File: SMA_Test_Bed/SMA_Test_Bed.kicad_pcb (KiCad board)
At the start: 2 copper layers, 108.6 x 58.3 mm, 157 parts, among them J1 Conn_02x14_Counter_Clockwise, J10 Conn_01x02_Socket, J11 Conn_01x02_Socket, J12 Conn_01x02_Socket, J13 Conn_01x02_Socket, J14 Conn_01x02_Socket, J15 Conn_01x02_Socket, J16 Conn_01x02_Socket, J17 Conn_01x02_Socket, J18 Conn_01x02_Socket, J2 Conn_01x02_Socket, J3 Conn_01x02_Socket, J4 Conn_01x02_Socket, J5 Conn_01x02_Socket, J6 Conn_01x02_Socket, J7 Conn_01x02_Socket, J8 Conn_01x02_Socket, J9 Conn_01x02_Socket, Q1 NMOS, Q10 NMOS, Q11 NMOS, Q12 NMOS, Q13 NMOS, Q14 NMOS, Q15 NMOS, Q16 NMOS, Q2 NMOS, Q3 NMOS, Q4 NMOS, Q5 NMOS, Q6 NMOS, Q7 NMOS, Q8 NMOS, Q9 NMOS, U1 PCA9685PW, U2 TLV9044, U3 TLV9044, U4 TLV9044, U5 TLV9044

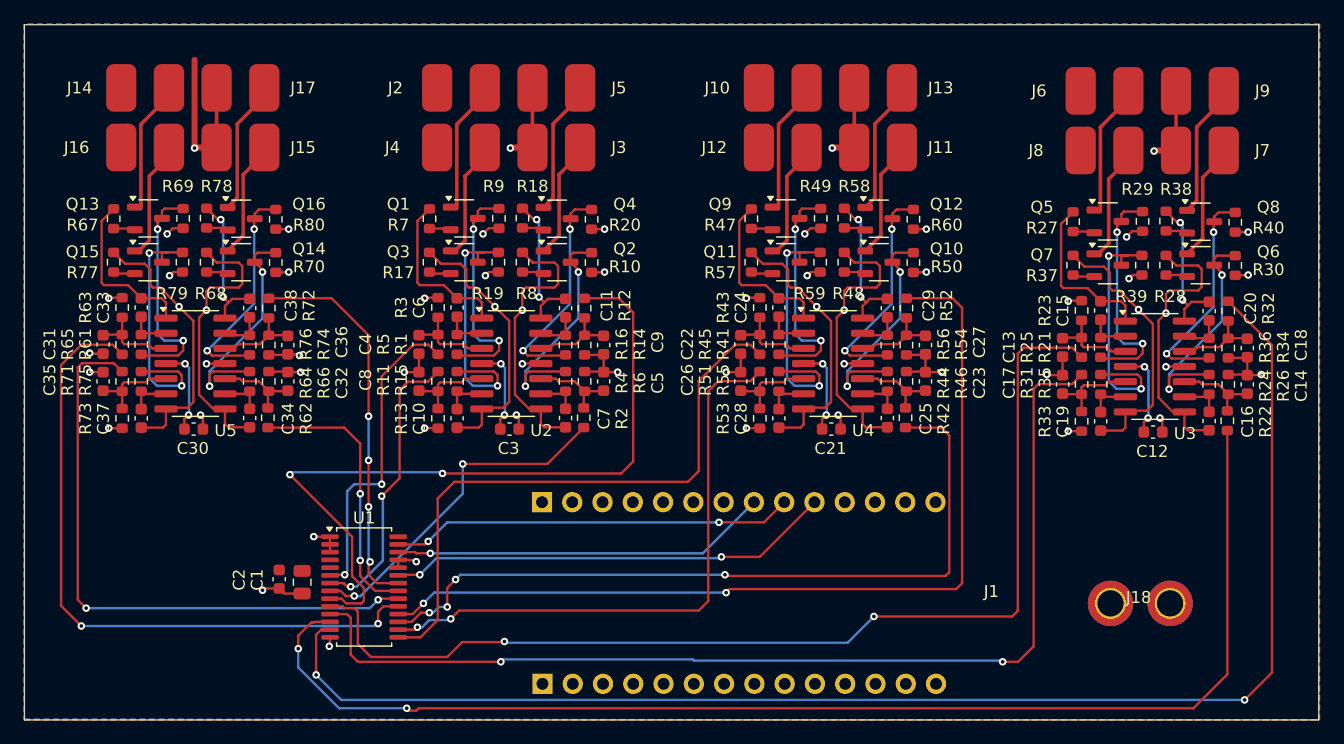
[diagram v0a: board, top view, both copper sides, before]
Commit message: Layout draft complete
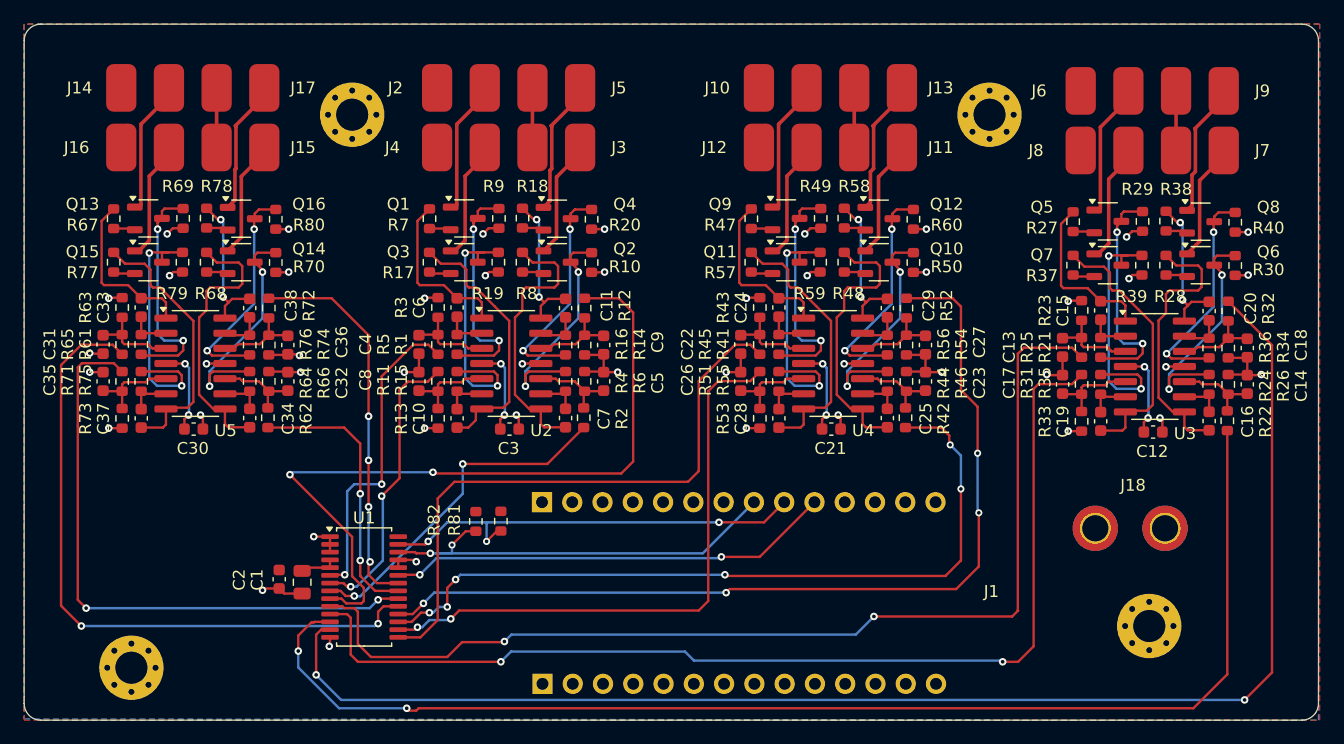
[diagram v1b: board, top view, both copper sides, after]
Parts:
- added H1: MountingHole, MountingHole:MountingHole_2.7mm_Pad_Via, F.Cu at (180.6, 79.5)
- added H2: MountingHole, MountingHole:MountingHole_2.7mm_Pad_Via, F.Cu at (127.1, 79.5)
- added H3: MountingHole, MountingHole:MountingHole_2.7mm_Pad_Via, F.Cu at (108.6, 125.9)
- added H4: MountingHole, MountingHole:MountingHole_2.7mm_Pad_Via, F.Cu at (194.0, 122.4)
- added R81: R_US, Resistor_SMD:R_0603_1608Metric, F.Cu at (137.5, 113.6)
- added R82: R_US, Resistor_SMD:R_0603_1608Metric, F.Cu at (139.6, 113.6)
- moved J18 6.43 mm to (191.8, 114.2)
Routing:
- net +3.3V: track 72.7 -> 61.0 mm, vias 12 -> 8
- net /SCL: track 31.7 -> 36.7 mm, vias 1 -> 2
- net /SDA: track 33.8 -> 37.1 mm, vias 2 -> 3
- net /bus2.PWM_SP3: track 76.5 -> 77.7 mm, vias 2 -> 4
- net /bus2.PWM_SP2: track 64.4 -> 65.2 mm, vias 4 -> 6
- net Net-(C10-Pad2): track 22.7 -> 21.9 mm, vias 1 -> 0
- net /bus1.PWM_SP1: track 89.3 -> 89.9 mm
- net Net-(C7-Pad2): vias 1 -> 0
- net Net-(C37-Pad2): vias 1 -> 0
- net Net-(C34-Pad2): vias 1 -> 0
- net Net-(C28-Pad2): vias 1 -> 0
- net Net-(C25-Pad2): vias 1 -> 0
- net Net-(C19-Pad2): vias 1 -> 0
- net Net-(C16-Pad2): vias 1 -> 0
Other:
- board size 108.6 x 58.3 mm -> 108.6 x 58.4 mm
